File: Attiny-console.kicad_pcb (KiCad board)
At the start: 2 copper layers, 30 x 40 mm, 15 parts, among them J1 SSD1306, J2 UDPI programming port, J3 Extra pins, SW1 SW_LEFT, SW2 SW_RIGHT, SW3 power_SW, SW4 power_SW, U1 ATtiny1616-S, U2 ATtiny1616-M

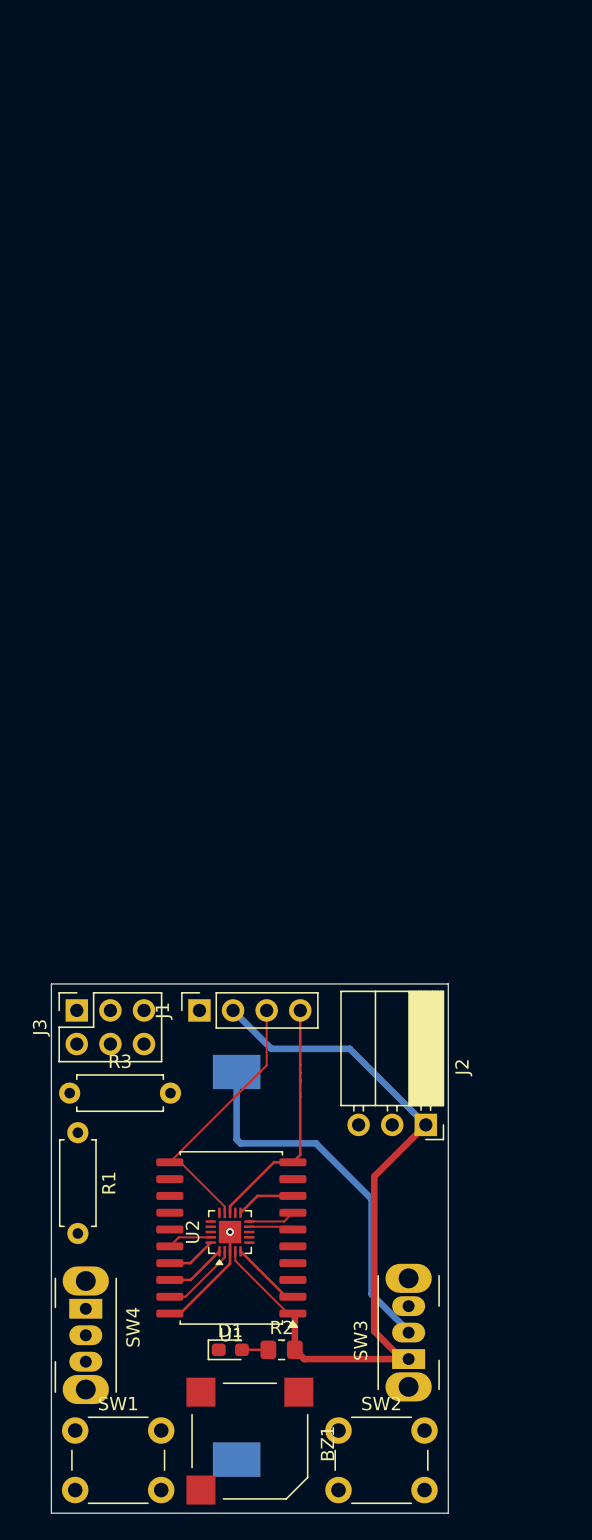
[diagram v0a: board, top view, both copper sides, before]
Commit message: Finishing the layout
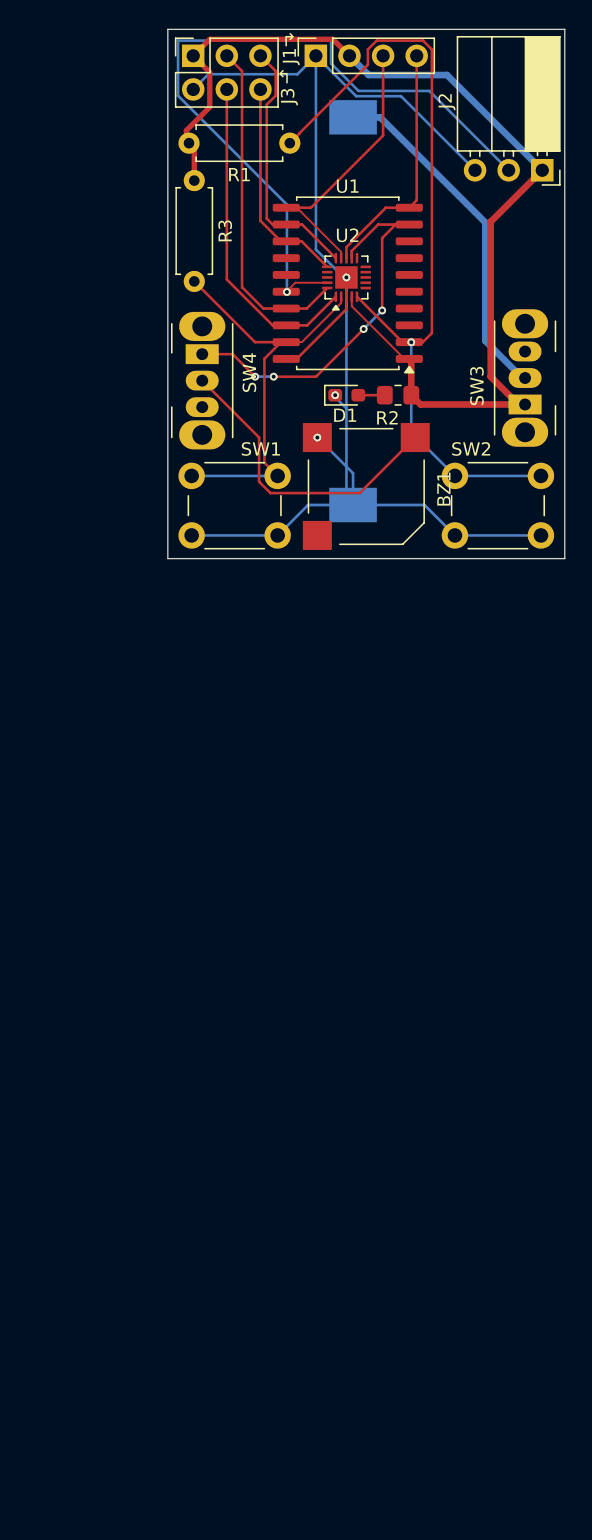
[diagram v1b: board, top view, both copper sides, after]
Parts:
- moved R1 75.3 mm to (35.4, 36.2), turned to 0 degrees
- moved BT1 72.7 mm to (47.8, 48.9)
- moved BZ1 72.7 mm to (48.8, 62.1)
- moved D1 72.7 mm to (47.3, 55.2)
- moved J1 72.7 mm to (45.0, 29.6)
- moved J2 72.7 mm to (62.1, 38.2)
- moved J3 72.7 mm to (35.7, 29.6)
- moved R2 72.7 mm to (51.2, 55.2)
- moved SW1 72.7 mm to (35.6, 61.4)
- moved SW2 72.7 mm to (55.5, 61.4)
- moved SW4 72.7 mm to (36.4, 52.1)
- moved U2 72.7 mm to (47.3, 46.4)
- moved SW3 72.7 mm to (60.8, 56.0)
- moved U1 72.7 mm to (47.4, 46.8)
- moved R3 69.6 mm to (35.8, 39.0), turned to -90 degrees
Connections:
- J3 pad 3: /pb4 -> /MOSI
- J3 pad 5: /pb5 -> /pc0
- J3 pad 6: /MOSI -> /pc1
- U1 pad 12: unconnected-(U1-PC0-Pad12) -> /pc0
- U1 pad 13: unconnected-(U1-PC1-Pad13) -> /pc1
- U1 pad 6: /pb5 -> unconnected-(U1-PB5-Pad6)
- U1 pad 7: /pb4 -> unconnected-(U1-PB4-Pad7)
- U1 pad 8: /buzz -> unconnected-(U1-PB3-Pad8)
- U1 pad 9: unconnected-(U1-PB2-Pad9) -> /buzz
- U2 pad 10: /pb4 -> unconnected-(U2-PB4-Pad10)
- U2 pad 11: /buzz -> unconnected-(U2-PB3-Pad11)
- U2 pad 12: unconnected-(U2-PB2-Pad12) -> /buzz
- U2 pad 15: unconnected-(U2-PC0-Pad15) -> /pc0
- U2 pad 16: unconnected-(U2-PC1-Pad16) -> /pc1
- U2 pad 9: /pb5 -> unconnected-(U2-PB5-Pad9)
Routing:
- net GND: track 8.51 -> 105.5 mm, vias 1 -> 3
- net /right: track 5.37 -> 61.5 mm, vias 0 -> 1
- net /UDPI: track 3.38 -> 55.9 mm, vias 0 -> 1
- net /left: track 6.26 -> 32.3 mm
- net /buzz: track 4.48 -> 30.1 mm, vias 0 -> 4
- net VCC: track 57.4 -> 81.3 mm
- net Net-(BZ1-+): track 0.00 -> 23.3 mm
- net /MOSI: track 3.74 -> 25.7 mm
- net /MISO: track 4.65 -> 24.9 mm
- net /pc0: track 0.00 -> 19.5 mm
- net /pc1: track 0.00 -> 16.4 mm
- net /pb4: track 3.57 -> 0.00 mm
- net /pb5: track 3.39 -> 0.00 mm
- net Net-(BT1-+): track 29.0 -> 26.9 mm
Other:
- board text added: "↰"
- board text added: "↱"
